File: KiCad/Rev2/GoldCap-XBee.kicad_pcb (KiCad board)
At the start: 4 copper layers, 34.7 x 55.6 mm, 30 parts, among them J1 5-7.5V, J2 3V3 IN, J3 VREF, J4 USART, Q1 BC847, Q2 IRLML6401, U1 LMV331

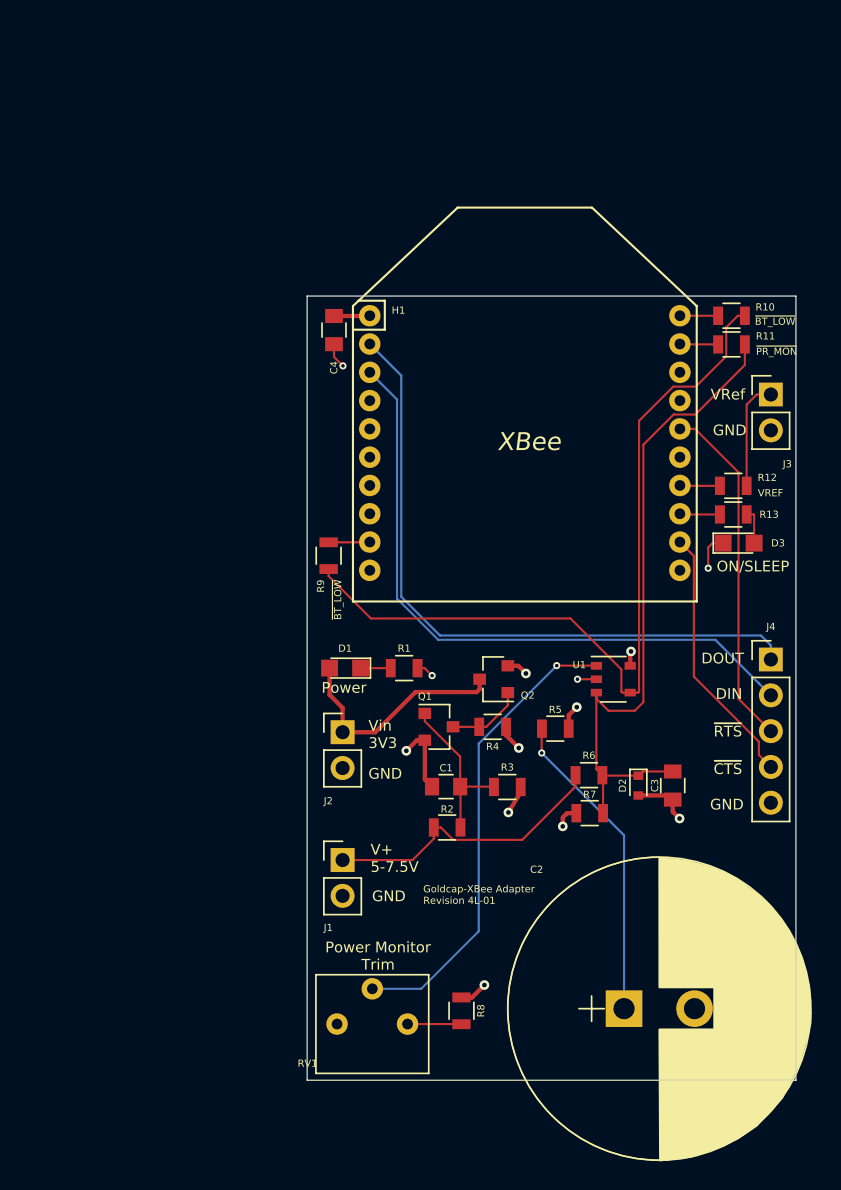
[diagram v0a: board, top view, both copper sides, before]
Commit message: Rev 2 of the dev board
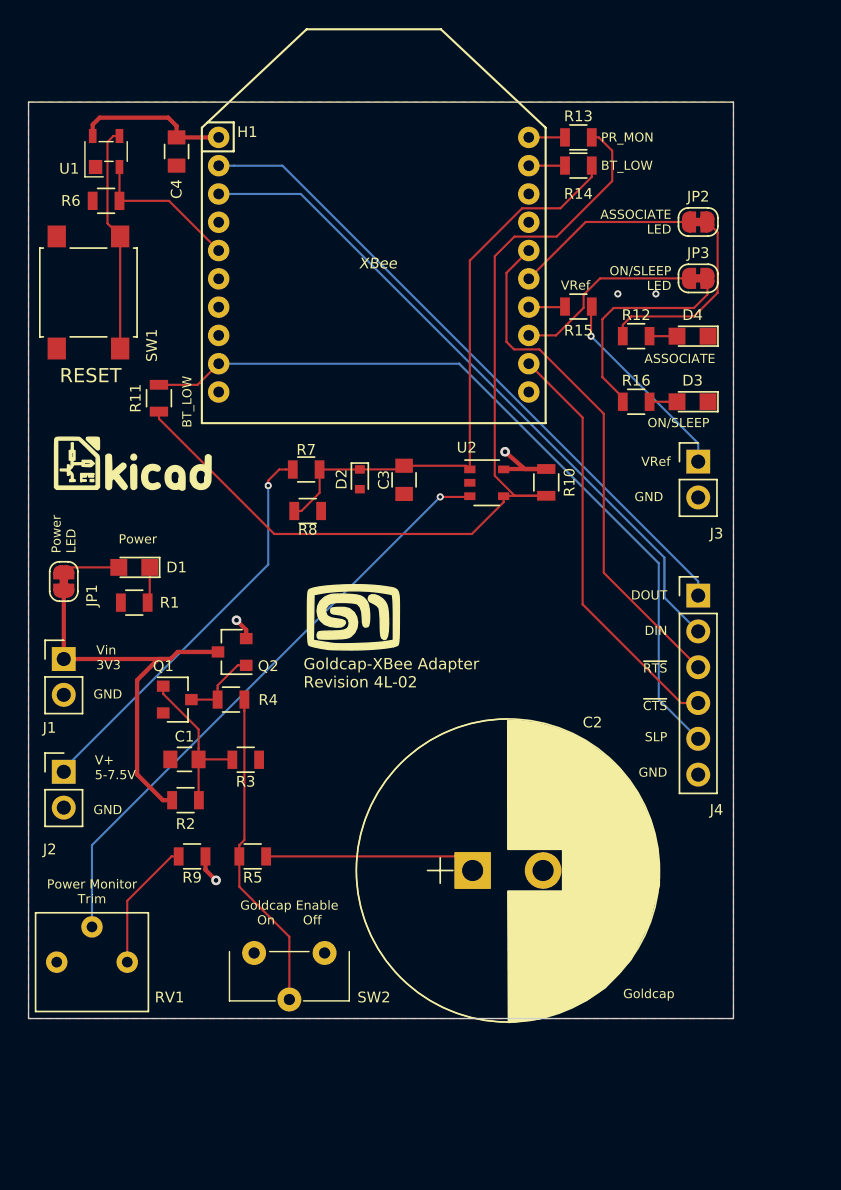
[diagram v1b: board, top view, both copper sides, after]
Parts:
- removed the G*** at (137.6, 83.3)
- added D4: LED, LEDs:LED_0805, F.Cu at (147.1, 66.6)
- added G***: LOGO, GoldCap-Check:MyBasic_rounded_50_1, B.Cu at (127.0, 75.5)
- added G***: LOGO, GoldCap-Check:KiCad-Logo, B.Cu at (143.2, 111.8)
- added G***: LOGO, GoldCap-Check:KiCad-Logo, F.Cu at (107.4, 75.6)
- added G***: LOGO, GoldCap-Check:MyBasic_rounded_50_1, F.Cu at (123.0, 86.5)
- added JP1: Pwr LED, Jumper:SolderJumper-2_P1.3mm_Bridged_RoundedPad1.0x1.5mm, F.Cu at (102.5, 84.0)
- added JP2: ASSOCIATE_BR, Jumper:SolderJumper-2_P1.3mm_Bridged_RoundedPad1.0x1.5mm, F.Cu at (147.5, 58.5)
- added JP3: ON, Jumper:SolderJumper-2_P1.3mm_Bridged_RoundedPad1.0x1.5mm, F.Cu at (147.5, 62.5)
- added R10: 10kΩ, Resistors_SMD:R_0805, F.Cu at (136.7, 77.0)
- added R12: 680Ω, Resistors_SMD:R_0805, F.Cu at (143.1, 66.6)
- added R6: 100kΩ, Resistors_SMD:R_0805, F.Cu at (105.5, 57.0)
- added SW1: Reset, Buttons_Switches_SMD:SW_SPST_B3S-1000, F.Cu at (104.2, 63.5)
- added SW2: SW_SPDT, GoldCap-Check:SPST-CL-SB-12C01, F.Cu at (118.5, 112.0)
- added U1: SGM811, GoldCap-Check:SGM811B, F.Cu at (105.5, 53.5)
- J4: value USART -> Conn_01x06_Female; footprint Pin_Headers:Pin_Header_Straight_1x05_Pitch2.54mm -> Pin_Headers:Pin_Header_Straight_1x06_Pitch2.54mm
- moved R7 29.5 mm to (119.7, 76.1)
- moved D2 29.4 mm to (123.5, 76.8)
- moved R8 29.3 mm to (119.8, 79.0), turned to 0 degrees
- moved C3 28.9 mm to (126.6, 76.8)
- moved R5 23.3 mm to (115.9, 103.5), turned to 0 degrees
- moved R9 22.0 mm to (111.6, 103.5), turned to 180 degrees
- moved J2 20.7 mm to (102.5, 97.5)
- moved J1 20.4 mm to (102.5, 89.5)
- moved RV1 20.4 mm to (104.5, 111.0)
- moved R1 19.7 mm to (107.5, 85.5), turned to 180 degrees
- moved Q1 18.7 mm to (110.6, 92.4)
- moved Q2 18.7 mm to (114.4, 89.0)
- moved R4 18.7 mm to (114.4, 92.4)
- moved C1 18.7 mm to (111.1, 96.6)
- moved R2 18.7 mm to (111.1, 99.5)
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- renumbered J2 to J1, J1 to J2, R9 to R11, R10 to R13, R11 to R14, R12 to R15, R13 to R16, R6 to R7, R7 to R8, R8 to R9, U1 to U2
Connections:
- net /ON_~SLEEP~ renamed /ON
- D1 pad 2: /VIN_3V3 -> Net-(D1-Pad2)
- H1 pad 15: (no net) -> Net-(H1-Pad15)
- H1 pad 5: (no net) -> /~RESET
- J4 pad 5: GND -> /SLEEP_REQ
- R16 pad 2: Net-(H1-Pad13) -> Net-(JP3-Pad2)
- R2 pad 2: /Vb -> /VIN_3V3
- R4 pad 2: /VCC -> Net-(R4-Pad2)
- R5 pad 1: /VCC -> Net-(R4-Pad2)
- U2 pad 1: /Vref -> /PWR_MON
- U2 pad 3: /PWR_MON -> /Vref
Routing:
- net /SLEEP_REQ: track 2.93 -> 55.5 mm
- net Net-(R4-Pad2): track 0.00 -> 22.9 mm
- net GND: track 20.0 -> 0.00 mm, vias 8 -> 2
- net Net-(SW1-Pad2): track 0.00 -> 16.1 mm
- net Net-(JP3-Pad2): track 0.00 -> 15.8 mm
- net Net-(JP2-Pad2): track 0.00 -> 13.8 mm
- net Net-(H1-Pad15): track 0.00 -> 13.0 mm
- net /VIN_3V3: track 16.6 -> 28.9 mm
- net /~XBEE_RTS: track 24.7 -> 36.9 mm
- net /~XBEE_CTS: track 18.6 -> 29.7 mm
- net /~RESET: track 0.00 -> 10.9 mm
- net Net-(H1-Pad13): track 2.86 -> 13.6 mm
- net /VCC: track 10.7 -> 21.0 mm, vias 5 -> 3
- net /Vref: track 33.2 -> 42.9 mm
- net /~BATT_LOW~: track 57.9 -> 67.1 mm
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- added copper zone on F.Cu, net GND
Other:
- board size 34.7 x 55.6 mm -> 50 x 65 mm
- rule pad_to_mask_clearance: 0.0508 -> 0
- board text added: "ASSOCIATE"
- board text added: "ASSOCIATE LED"
- board text added: "BT_LOW"
- board text added: "Goldcap"
- board text added: "Goldcap Enable On Off"
- board text added: "Goldcap-XBee Adapter Revision 4L-02"
- board text added: "ON/SLEEP LED"
- board text added: "PR_MON"
- board text added: "Power LED"
- board text added: "RESET"
- board text added: "SLP"
- board text removed: "Goldcap-XBee Adapter Revision 4L-01"
- board text removed: "VREF"
- board text removed: "~BT_LOW~"
- board text removed: "~PR_MON~"
